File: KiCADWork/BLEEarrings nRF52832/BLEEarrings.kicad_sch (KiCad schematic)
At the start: 3 parts, among them J3 USB_C_Receptacle, SW1 TK-6580B-1

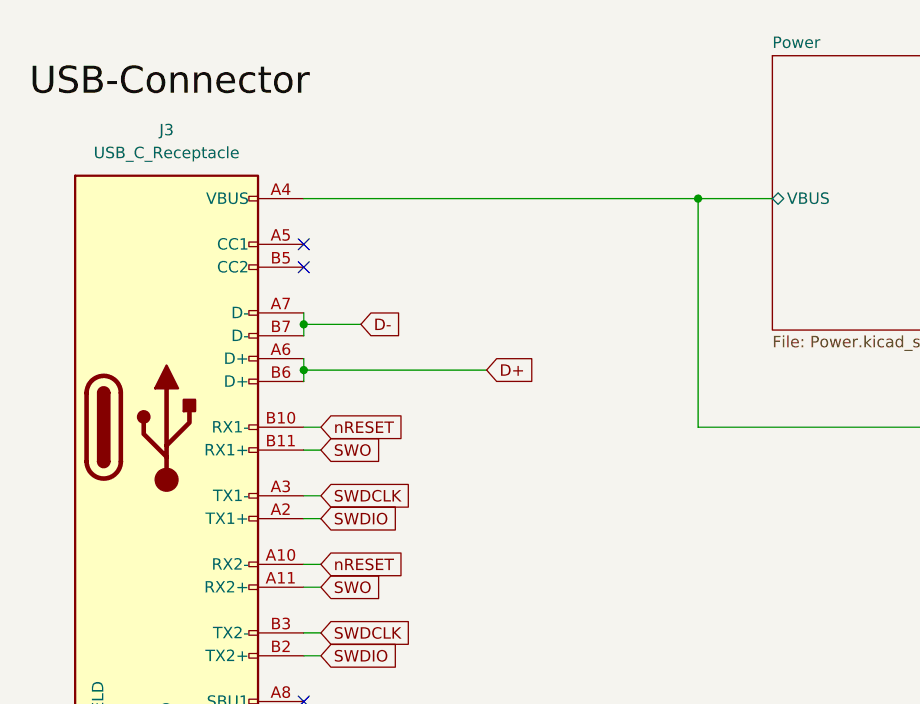
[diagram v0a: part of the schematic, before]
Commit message: Dock Updates
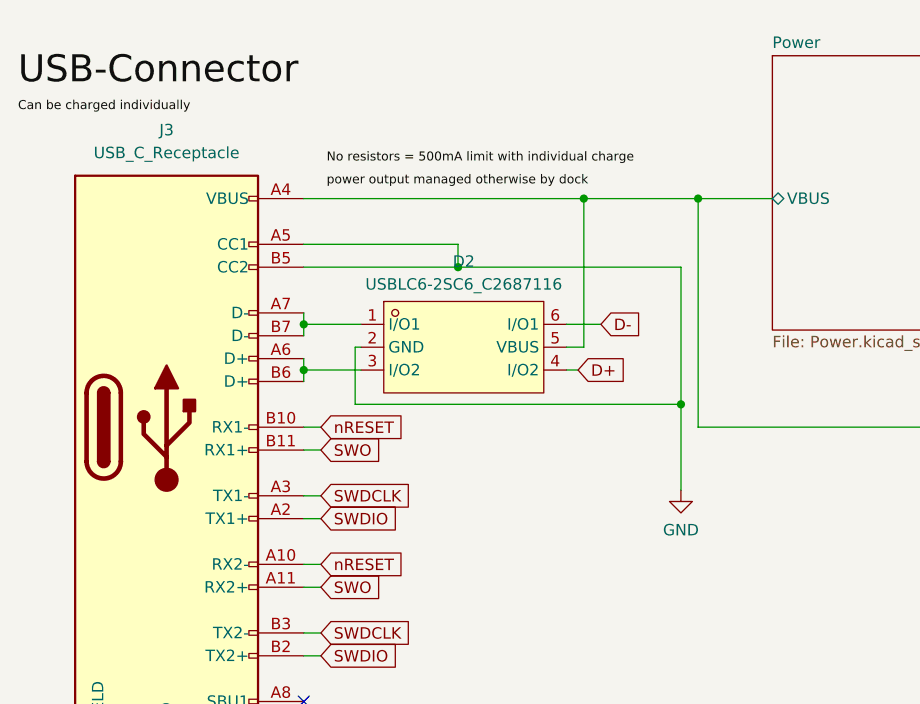
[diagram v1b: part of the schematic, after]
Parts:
- added D2: USBLC6-2SC6_C2687116, easyeda2kicad:SOT-23-6_L2.9-W1.6-P0.95-LS2.8-BL, symbol easyeda2kicad:USBLC6-2SC6_C2687116
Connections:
- net D+: now also D2.4 (I/O2); no longer J3.A6 (D+), J3.B6 (D+)
- net D-: now also D2.6 (I/O1); no longer J3.A7 (D-), J3.B7 (D-)
- net DSP/VBUS: now also D2.5 (VBUS)
- net GND: now also J3.A5 (CC1), J3.B5 (CC2), D2.2 (GND)
- new net: D2.1 (I/O1), J3.A7 (D-), J3.B7 (D-)
- new net: D2.3 (I/O2), J3.A6 (D+), J3.B6 (D+)
- no-connect marks 4 -> 2
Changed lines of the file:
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@@
   (junction (at 92.075 88.265) (diameter 0) (color 0 0 0 0)
   )
+  (junction (at 109.22 76.835) (diameter 0) (color 0 0 0 0)
+  )
+  (junction (at 133.985 92.075) (diameter 0) (color 0 0 0 0)
+  )
   (junction (at 92.075 83.185) (diameter 0) (color 0 0 0 0)
   )
@@
   )
   (junction (at 210.185 68.58) (diameter 0) (color 0 0 0 0)
+  )
+  (junction (at 123.19 69.215) (diameter 0) (color 0 0 0 0)
   )
   (no_connect (at 92.075 127.635))
   (no_connect (at 92.075 125.095))
-  (no_connect (at 92.075 76.835))
-  (no_connect (at 92.075 74.295))
   (wire (pts (xy 191.135 112.395) (xy 196.215 112.395))
     (stroke (width 0) (type default))
   )
+  (wire (pts (xy 92.075 74.295) (xy 109.22 74.295))
+    (stroke (width 0) (type default))
+  )
+  (wire (pts (xy 109.22 74.295) (xy 109.22 76.835))
+    (stroke (width 0) (type default))
+  )
   (wire (pts (xy 222.25 68.58) (xy 243.84 68.58))
     (stroke (width 0) (type default))
@@
     (stroke (width 0) (type default))
   )
+  (wire (pts (xy 121.285 83.185) (xy 125.095 83.185))
+    (stroke (width 0) (type default))
+  )
   (wire (pts (xy 93.98 102.235) (xy 92.075 102.235))
     (stroke (width 0) (type default))
   )
+  (wire (pts (xy 121.285 88.265) (xy 122.555 88.265))
+    (stroke (width 0) (type default))
+  )
   (wire (pts (xy 93.98 117.475) (xy 92.075 117.475))
     (stroke (width 0) (type default))
   )
+  (wire (pts (xy 97.79 85.725) (xy 97.79 92.075))
+    (stroke (width 0) (type default))
+  )
   (wire (pts (xy 222.25 68.58) (xy 222.25 73.025))
     (stroke (width 0) (type default))
@@
     (stroke (width 0) (type default))
   )
+  (wire (pts (xy 133.985 92.075) (xy 133.985 101.6))
+    (stroke (width 0) (type default))
+  )
   (wire (pts (xy 73.025 135.255) (xy 76.835 135.255))
     (stroke (width 0) (type default))
@@
     (stroke (width 0) (type default))
   )
+  (wire (pts (xy 133.985 92.075) (xy 133.985 76.835))
+    (stroke (width 0) (type default))
+  )
   (wire (pts (xy 135.89 69.215) (xy 144.145 69.215))
     (stroke (width 0) (type default))
@@
     (stroke (width 0) (type default))
   )
-  (wire (pts (xy 92.075 88.265) (xy 112.395 88.265))
+  (wire (pts (xy 92.075 88.265) (xy 98.425 88.265))
+    (stroke (width 0) (type default))
+  )
+  (wire (pts (xy 123.19 69.215) (xy 123.19 85.725))
     (stroke (width 0) (type default))
   )
@@
     (stroke (width 0) (type default))
   )
-  (wire (pts (xy 92.075 69.215) (xy 135.89 69.215))
+  (wire (pts (xy 92.075 69.215) (xy 123.19 69.215))
     (stroke (width 0) (type default))
   )
@@
     (stroke (width 0) (type default))
   )
+  (wire (pts (xy 92.075 76.835) (xy 109.22 76.835))
+    (stroke (width 0) (type default))
+  )
+  (wire (pts (xy 123.19 69.215) (xy 135.89 69.215))
+    (stroke (width 0) (type default))
+  )
   (wire (pts (xy 92.075 81.915) (xy 92.075 83.185))
     (stroke (width 0) (type default))
@@
     (stroke (width 0) (type default))
   )
+  (wire (pts (xy 98.425 85.725) (xy 97.79 85.725))
+    (stroke (width 0) (type default))
+  )
   (wire (pts (xy 191.135 125.73) (xy 196.215 125.73))
     (stroke (width 0) (type default))
@@
   )
   (wire (pts (xy 73.025 138.43) (xy 73.025 135.255))
+    (stroke (width 0) (type default))
+  )
+  (wire (pts (xy 109.22 76.835) (xy 133.985 76.835))
+    (stroke (width 0) (type default))
+  )
+  (wire (pts (xy 97.79 92.075) (xy 133.985 92.075))
+    (stroke (width 0) (type default))
+  )
+  (wire (pts (xy 121.285 85.725) (xy 123.19 85.725))
     (stroke (width 0) (type default))
   )
@@
     (effects (font (size 1 1)) (justify left bottom))
   )
+  (label "Can be charged individually" (at 60.325 59.69 0) (fields_autoplaced)
+    (effects (font (size 1 1)) (justify left bottom))
+  )
   (label "PWR Switch" (at 202.565 54.61 0) (fields_autoplaced)
     (effects (font (size 3 3)) (justify left bottom))
   )
-  (label "USB-Connector" (at 61.595 58.42 0) (fields_autoplaced)
+  (label "USB-Connector" (at 60.325 57.15 0) (fields_autoplaced)
     (effects (font (size 3 3)) (justify left bottom))
   )
+  (label "No resistors = 500mA limit with individual charge" (at 94.615 65.405 0) (fields_autoplaced)
+    (effects (font (size 1 1)) (justify left bottom))
+  )
+  (label "power output managed otherwise by dock" (at 94.615 67.945 0) (fields_autoplaced)
+    (effects (font (size 1 1)) (justify left bottom))
+  )
   (global_label "D-" (shape input) (at 191.135 122.555 180) (fields_autoplaced)
     (effects (font (size 1.27 1.27)) (justify right))
@@
     )
   )
-  (global_label "D+" (shape input) (at 112.395 88.265 0) (fields_autoplaced)
-    (effects (font (size 1.27 1.27)) (justify left))
-    (property "Intersheetrefs" "${INTERSHEET_REFS}" (at 118.2226 88.265 0)
+  (global_label "D+" (shape input) (at 122.555 88.265 0) (fields_autoplaced)
+    (effects (font (size 1.27 1.27)) (justify left))
+    (property "Intersheetrefs" "${INTERSHEET_REFS}" (at 128.3826 88.265 0)
       (effects (font (size 1.27 1.27)) (justify left) hide)
     )
@@
     )
   )
-  (global_label "D-" (shape input) (at 98.425 83.185 0) (fields_autoplaced)
-    (effects (font (size 1.27 1.27)) (justify left))
-    (property "Intersheetrefs" "${INTERSHEET_REFS}" (at 104.2526 83.185 0)
+  (global_label "D-" (shape input) (at 125.095 83.185 0) (fields_autoplaced)
+    (effects (font (size 1.27 1.27)) (justify left))
+    (property "Intersheetrefs" "${INTERSHEET_REFS}" (at 130.9226 83.185 0)
       (effects (font (size 1.27 1.27)) (justify left) hide)
     )
@@
         (path "/fde3e4b3-cb63-4f5f-903c-f7733537b674"
           (reference "SW1") (unit 1)
+        )
+      )
+    )
+  )
+  (symbol (lib_id "easyeda2kicad:USBLC6-2SC6_C2687116") (at 109.855 85.725 0) (unit 1)
+    (in_bom yes) (on_board yes) (dnp no) (fields_autoplaced)
+    (property "Reference" "D2" (at 109.855 76.2 0)
+      (effects (font (size 1.27 1.27)))
+    )
+    (property "Value" "USBLC6-2SC6_C2687116" (at 109.855 78.74 0)
+      (effects (font (size 1.27 1.27)))
+    )
+    (property "Footprint" "easyeda2kicad:SOT-23-6_L2.9-W1.6-P0.95-LS2.8-BL" (at 109.855 95.885 0)
+      (effects (font (size 1.27 1.27)) hide)
+    )
+    (property "Datasheet" "" (at 109.855 85.725 0)
+      (effects (font (size 1.27 1.27)) hide)
+    )
+    (property "LCSC Part" "C2687116" (at 109.855 98.425 0)
+      (effects (font (size 1.27 1.27)) hide)
+    )
+    (pin "6")
+    (pin "3")
+    (pin "4")
+    (pin "2")
+    (pin "1")
+    (pin "5")
+    (instances
+      (project "BLEEarrings"
+        (path "/fde3e4b3-cb63-4f5f-903c-f7733537b674"
+          (reference "D2") (unit 1)
         )
       )
@@
         )
       )
+    )
+  )
+  (symbol (lib_id "power:GND") (at 133.985 101.6 0) (unit 1)
+    (in_bom yes) (on_board yes) (dnp no) (fields_autoplaced)
+    (property "Reference" "#PWR023" (at 133.985 107.95 0)
+      (effects (font (size 1.27 1.27)) hide)
+    )
+    (property "Value" "GND" (at 133.985 106.045 0)
+      (effects (font (size 1.27 1.27)))
+    )
+    (property "Footprint" "" (at 133.985 101.6 0)
+      (effects (font (size 1.27 1.27)) hide)
+    )
+    (property "Datasheet" "" (at 133.985 101.6 0)
+      (effects (font (size 1.27 1.27)) hide)
+    )
+    (pin "1")
+    (instances
+      (project "BLEEarrings"
+        (path "/fde3e4b3-cb63-4f5f-903c-f7733537b674"
+          (reference "#PWR023") (unit 1)
+        )
+      )
